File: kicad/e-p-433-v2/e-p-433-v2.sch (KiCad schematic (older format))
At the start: 20 parts, among them P3 ant, P5 Transmitter, SW1 Capuchon vert, SW2 SW_PUSH_m, U3 Teensy_3-2

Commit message: Modification des fichiers e-p-433-v2.*
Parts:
- removed P?: Transmitter, Connect:PINHEAD1-6, symbol e-p-433-v2-rescue:CONN_01X06
- added J?: 2 X thermomètre digital, symbol Connector_Generic:Conn_01x08
- added R? (x2): 47K, symbol Device:R
- added R?: 1 OHM, symbol Device:R
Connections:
- net labels added: VBAT1
- net labels removed: VBAT
- wire segments 53 -> 75
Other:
- note added: "2 X DS 18B 2O"
- note added: "DQ"
- note added: "Entretoise de fixation [16]"
- note added: "Interface des thermomètres digitaux"
- note added: "Méplat"
- note added: "T1 -> Teensy 3.2 (D17)"
- note added: "T2 -> Teensy 3.2 (D16)"
- note added: "VDD"
- note added: "batterie"
- note added: "couvercle"
- moved on the sheet: C5, D1, D3, D4, P3, P5, R10, R11, R12, R13, R14, R16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

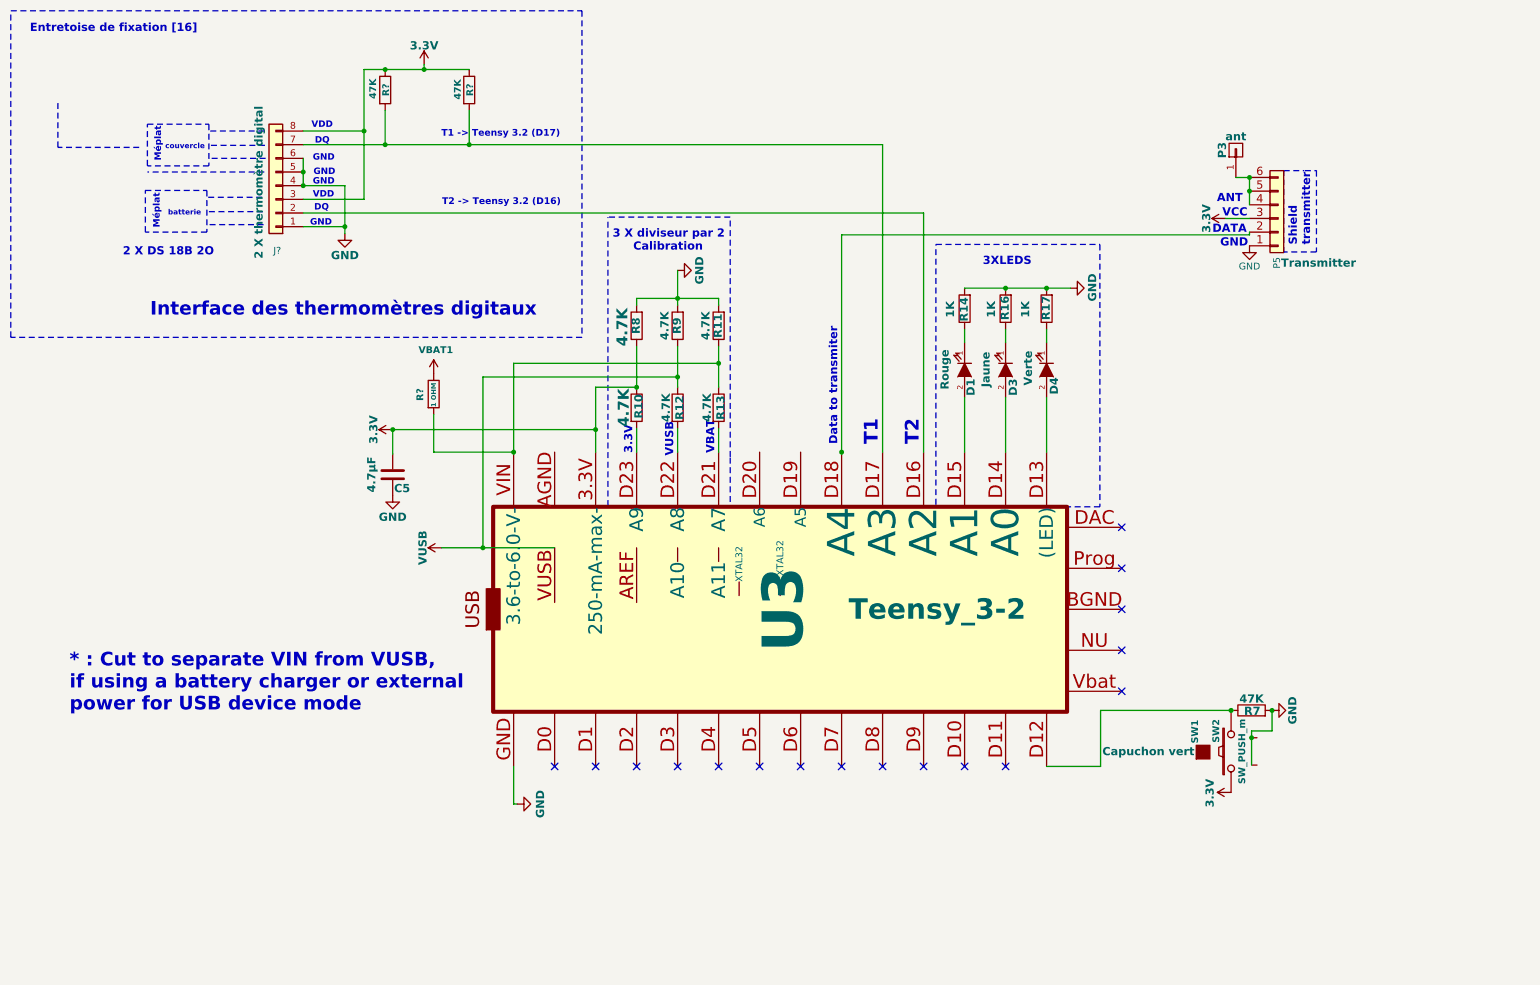
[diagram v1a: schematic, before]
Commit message: Reprise de kicad
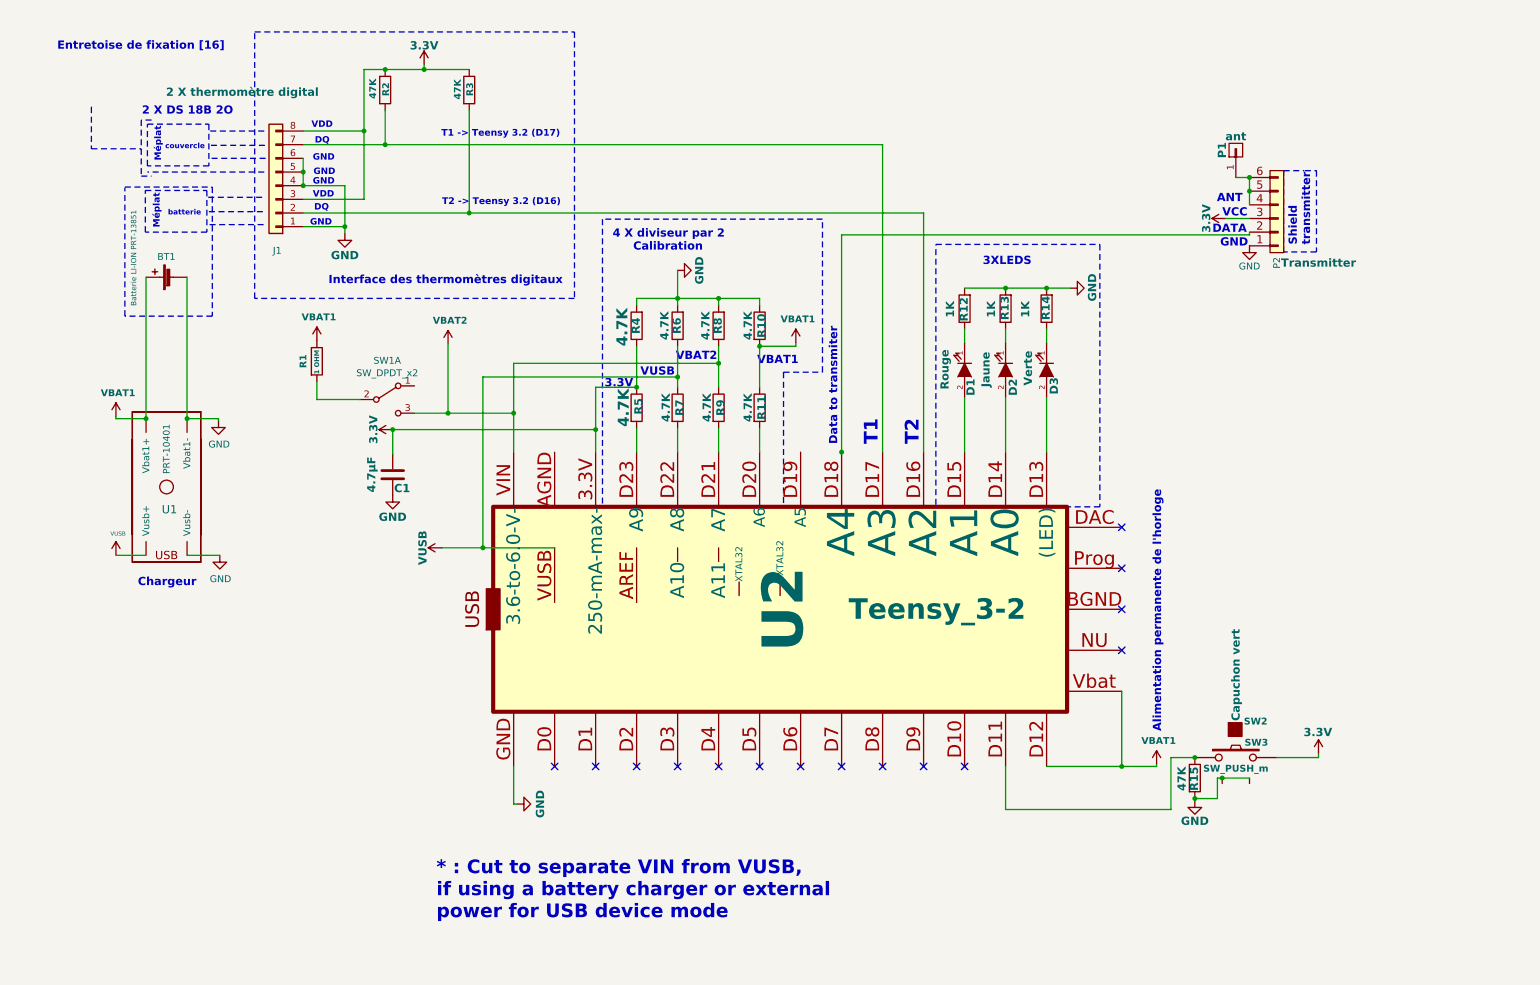
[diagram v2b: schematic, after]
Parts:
- added BT1: Batterie LI-ION PRT-13851, symbol Device:Battery_Cell
- added R10, R11: 4.7K, Resistors_SMD:R_0603, symbol e-p-433-v2-rescue:R
- added SW1: SW_DPDT_x2, symbol Switch:SW_DPDT_x2
- added U1: PRT-10401, symbol Sp:PRT-10401
- gave numbers to parts that had none: 4
- renumbered C5 to C1, D3 to D2, D4 to D3, P3 to P1, P5 to P2, R14 to R12, R16 to R13, R17 to R14, R7 to R15, R8 to R4, R10 to R5, R9 to R6, R12 to R7, R11 to R8, R13 to R9, SW1 to SW2, SW2 to SW3, U3 to U2
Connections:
- net +5V: now also U1.~ (Vusb-)
- net +BATT: now also R8.1, R9.1, U2.D12, U2.VIN (3.6-to-6.0-V-), U2.Vbat, BT1.1 (+), R10.2, R11.1, SW1.3 (C), U1.~ (Vusb-)
- net 3.3V: now also SW3.2; no longer SW3.1
- net GND: now also BT1.2 (-), R10.1, U1.~ (Vusb-)
- net at U2.D11: now also R15.1, SW3.1
- net at J1.2 (Pin_2), U2.D16 (A2): now also R3.2
- net at J1.7 (Pin_7), R2.2, U2.D17 (A3): no longer R3.2
- net at U2.D20 (A6): now also R11.2
- new net: R1.2, SW1.2 (B)
- no-connect marks 17 -> 15
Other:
- note added: "4 X diviseur par 2"
- note added: "Alimentation permanente de l'horloge"
- note added: "Chargeur"
- note added: "VBAT1"
- note added: "VBAT2"
- note removed: "3 X diviseur par 2"
- note removed: "VBAT"
- moved on the sheet: R1, R15, SW2, SW3

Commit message: Mise à jour de fichiers Kicad
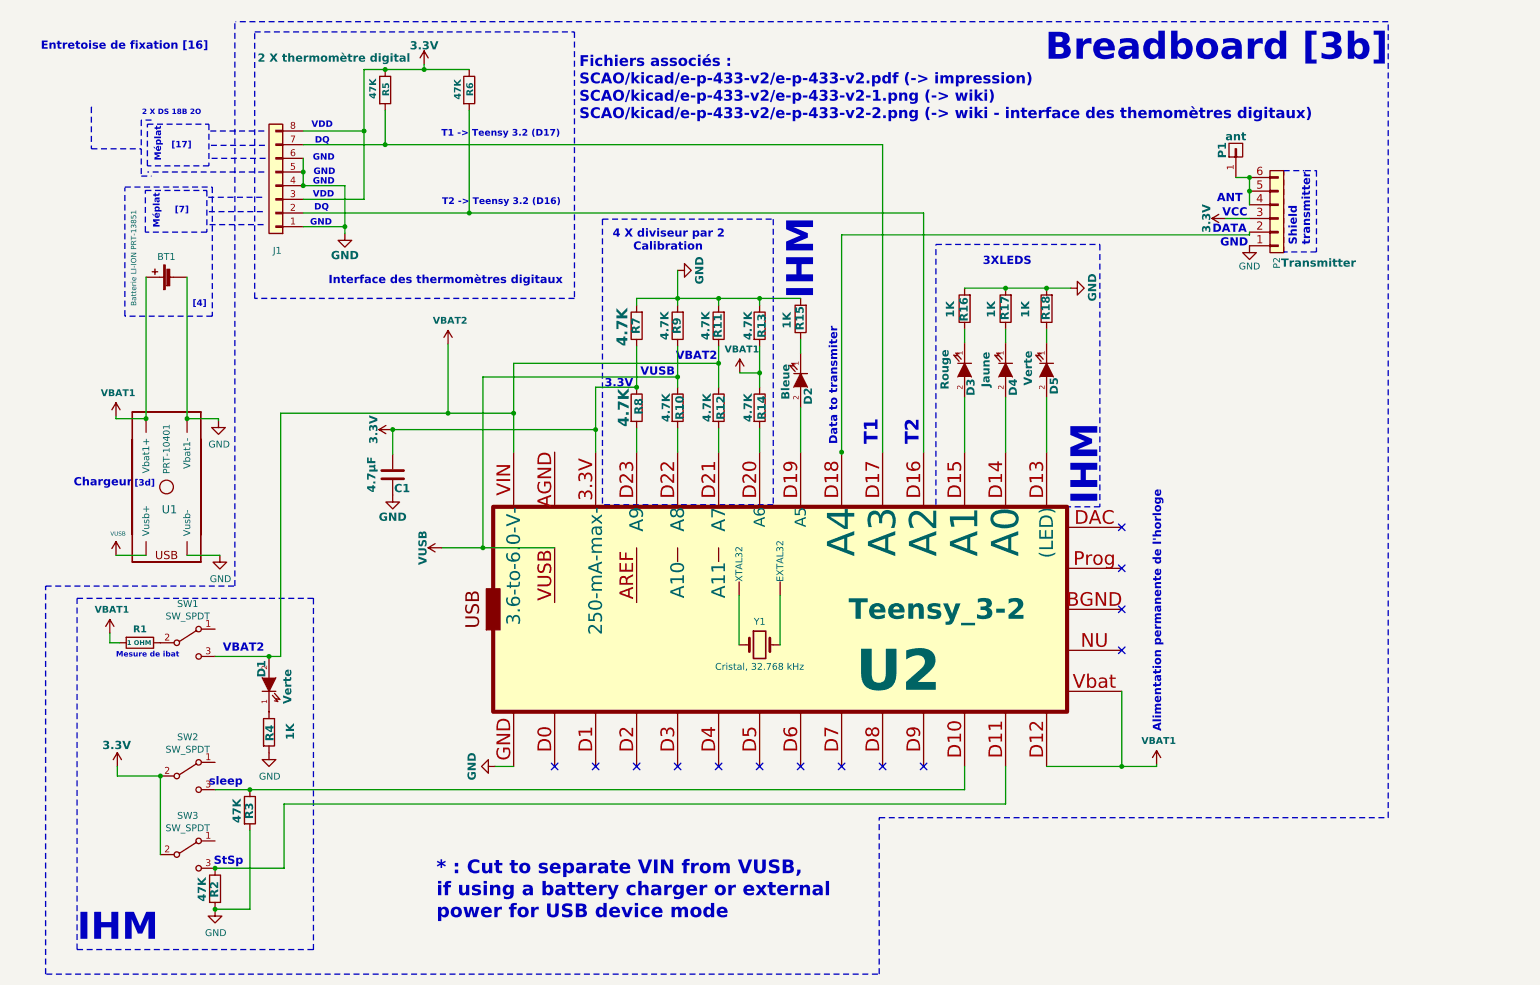
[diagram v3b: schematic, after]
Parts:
- removed SW1: SW_DPDT_x2, symbol Switch:SW_DPDT_x2
- removed SW2: Capuchon vert, Sp:Capuchon, symbol Sp:Capuchon
- removed SW3: SW_PUSH_m, Sp:SW_Micro_SPST_Angled, symbol Sp:SW_PUSH_m
- added D1: Verte, LEDs:LED_0603, symbol e-p-433-v2-rescue:LED-RESCUE-e-p-433-v2
- added D2: Bleue, LEDs:LED_0603, symbol e-p-433-v2-rescue:LED-RESCUE-e-p-433-v2
- added R2, R3: 47K, Resistors_SMD:R_0603, symbol e-p-433-v2-rescue:R
- added R4: 1K, Resistors_SMD:R_0603, symbol e-p-433-v2-rescue:R
- added SW1, SW2, SW3: SW_SPDT, symbol Switch:SW_SPDT
- added Y1: Cristal, 32.768 kHz, symbol Device:Crystal
- R15: value 47K -> 1K; Distributeur CONRAD -> Conrad; Désignation Résistance à couche épaisse 47 kΩ CMS 0603 0.1 W 5 % 100 ±p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 -> Résistance à couche épaisse 1 kΩ CMS 0603 0.1 W 5 %; Ref-distri 1457808 - 62 -> 1457724 - 62; Ref-fab 0603SAJ0473T5E -> 0603SAJ0102T5E
- renumbered D1 to D3, D2 to D4, D3 to D5, R7 to R10, R8 to R11, R9 to R12, R10 to R13, R11 to R14, R12 to R16, R13 to R17, R14 to R18, R2 to R5, R3 to R6, R4 to R7, R5 to R8, R6 to R9
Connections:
- net +BATT: now also R1.2, D1.2 (A), SW1.3 (C); no longer R1.1
- net 3.3V: now also SW2.2 (B), SW3.2 (B)
- net GND: now also R2.2, R3.2, R4.2
- net at U2.D10: now also R3.1, SW2.3 (C)
- net at U2.D11: now also R2.1, SW3.3 (C); no longer R15.1
- net at U2.D19 (A5): now also D2.2 (A)
- net at U2.~ (XTAL32): now also Y1.2
- new net: U2.~ (XTAL32), Y1.1
- new net: R1.1, SW1.2 (B)
- new net: D2.1 (K), R15.1
- new net: D1.1 (K), R4.1
- no-connect marks 15 -> 14
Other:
- note added: "Breadboard [3b]"
- note added: "Fichiers associés :\nSCAO/kicad/e-p-433-v2/e-p-433-v2.pdf (-> impression)\nSCAO/kicad/e-p-433-v2/e-p-433-v2-1.png (-> wiki)\nSCAO/kicad/e-p-433-v2/e-p-433-v2-2.png (-> wiki - interface des themomètres digitaux)"
- note added: "IHM"
- note added: "Mesure de ibat"
- note added: "StSp"
- note added: "[17]"
- note added: "[3d]"
- note added: "[4]"
- note added: "[7]"
- note added: "sleep"
- note removed: "VBAT1"
- note removed: "batterie"
- note removed: "couvercle"
- moved on the sheet: R1
